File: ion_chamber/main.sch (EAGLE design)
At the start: 7 parts, among them Q1 SST201

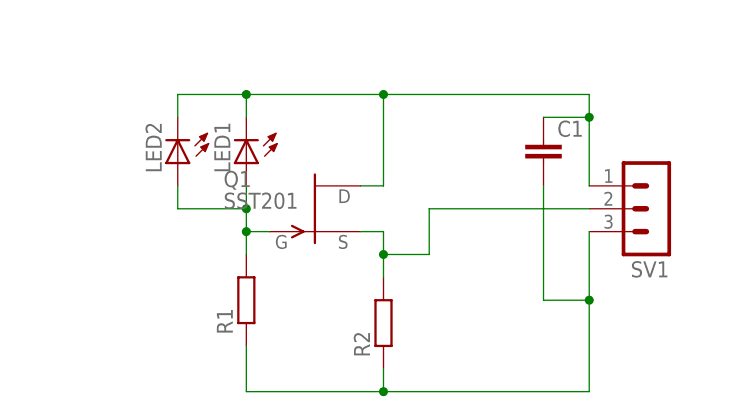
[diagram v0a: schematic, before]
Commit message: Output files added.
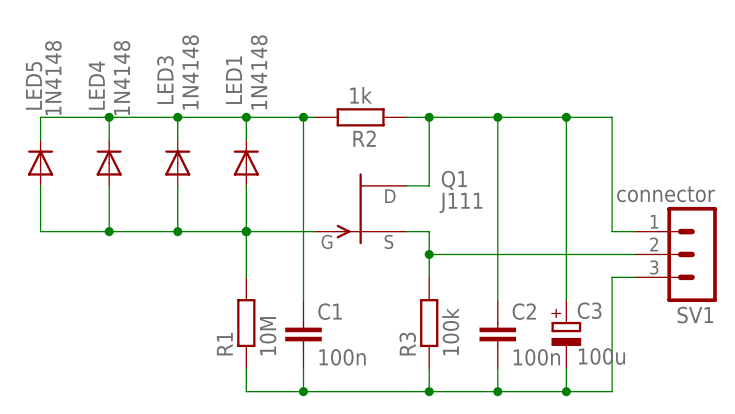
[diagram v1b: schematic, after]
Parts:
- removed LED2: (no value), led:LEDSFH480
- added C2: 100n, resistor:C-EUC1206
- added C3: 100u, resistor:CPOL-EUSMCC
- added LED3, LED4, LED5: 1N4148, diode:1N4148DO35-7
- added R3: 100k, resistor:R-EU_R1206
- C1: value (none) -> 100n; device resistor:C-EU025-050X050 -> resistor:C-EUC1206
- LED1: value (none) -> 1N4148; device led:LEDSFH480 -> diode:1N4148DO35-7
- Q1: value SST201 -> J111
- R1: value (none) -> 10M; device resistor:R-EU_0204/7 -> resistor:R-EU_0207/10
- R2: value (none) -> 1k; device resistor:R-EU_0204/7 -> resistor:R-EU_R1206
- SV1: value (none) -> connector
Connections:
- removed net N$3: C1.2, R1.1, R2.1, SV1.3
- new net GND: C1.2, C2.2, C3.-, R1.1, R3.1, SV1.3
- new net N$1: C1.1, LED1.C, LED3.C, LED4.C, LED5.C, R2.2
- net N$2: now also R3.2; no longer R2.2
- net N$4: now also LED3.A, LED4.A, LED5.A; no longer LED2.A
- net N$6: now also C2.1, C3.+, R2.1; no longer C1.1, LED1.C, LED2.C
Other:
- moved on the sheet: C1, Q1, R1, R2, SV1
